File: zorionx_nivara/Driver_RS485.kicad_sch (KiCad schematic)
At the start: 0 parts

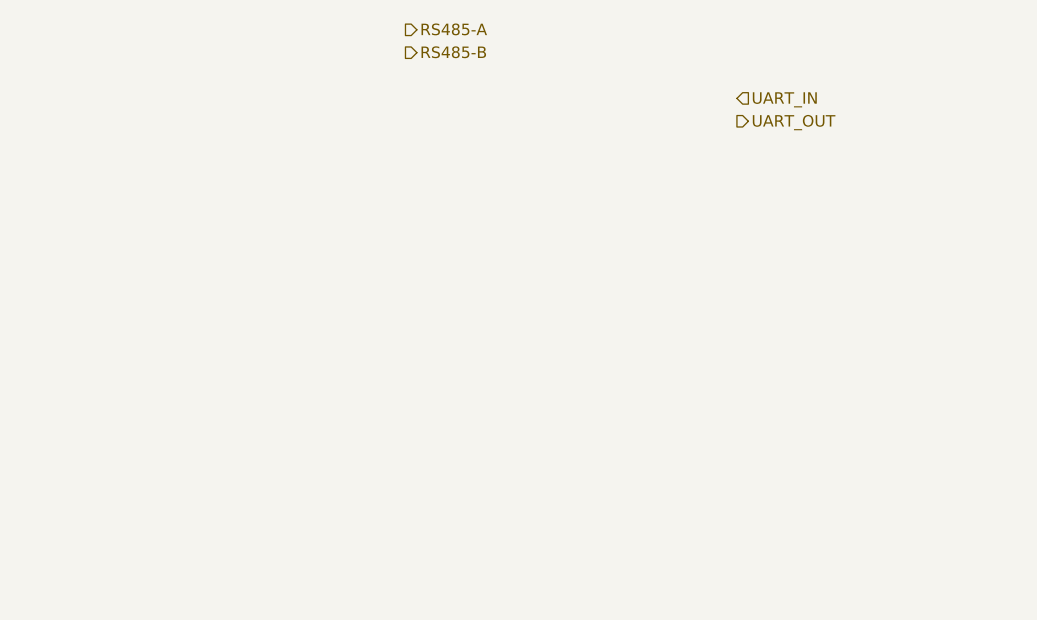
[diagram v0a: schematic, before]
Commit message: ultimo commit 1
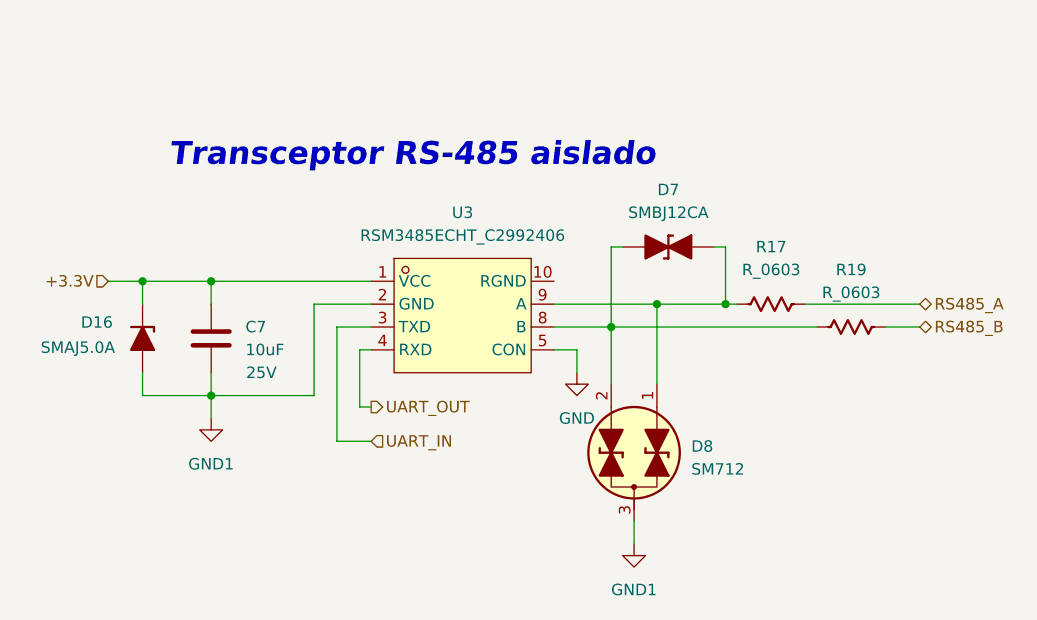
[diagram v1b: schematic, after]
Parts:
- added C7: 10uF, PCM_Capacitor_SMD_AKL:C_0603_1608Metric, symbol PCM_Capacitor_US_AKL:C_0603
- added D16: SMAJ5.0A, PCM_Diode_SMD_AKL:D_SMA, symbol PCM_Diode_TVS_AKL:SMAJ5.0A
- added D7: SMBJ12CA, PCM_Diode_SMD_AKL:D_SMB_TVS, symbol PCM_Diode_TVS_AKL:SMBJ12CA
- added D8: SM712, PCM_Package_TO_SOT_SMD_AKL:SOT-23, symbol PCM_Diode_TVS_AKL:SM712
- added R17, R19: R_0603, PCM_Resistor_SMD_AKL:R_0603_1608Metric, symbol PCM_Resistor_US_AKL:R_0603
- added U3: RSM3485ECHT_C2992406, EasyEDA:COMM-TH_8P-L19.5-W16.5-P2.54-BL, symbol EasyEDA:RSM3485ECHT_C2992406
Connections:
- net UART_IN: now also U3.3 (TXD)
- net UART_OUT: now also U3.4 (RXD)
- new net: D7.2 (A), D8.1 (A1), R17.1, U3.9 (A)
- new net: D7.1 (K), D8.2 (A2), R19.1, U3.8 (B)
- new net +3.3V: C7.1, D16.1 (K), U3.1 (VCC)
- new net GND: U3.5 (CON)
- new net GND1: C7.2, D16.2 (A), D8.3 (Com), U3.2 (GND)
- new net RS485_A: R17.2
- new net RS485_B: R19.2
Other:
- note added: "Transceptor RS-485 aislado"
